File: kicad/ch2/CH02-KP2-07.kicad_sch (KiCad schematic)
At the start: 5 parts

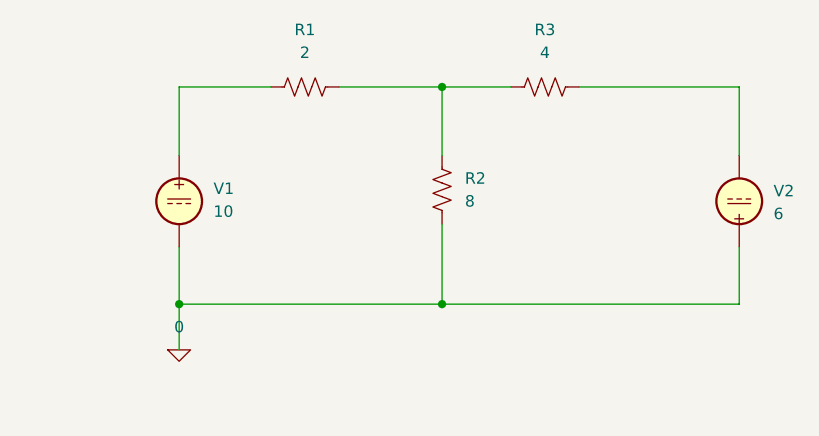
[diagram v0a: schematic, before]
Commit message: regular update
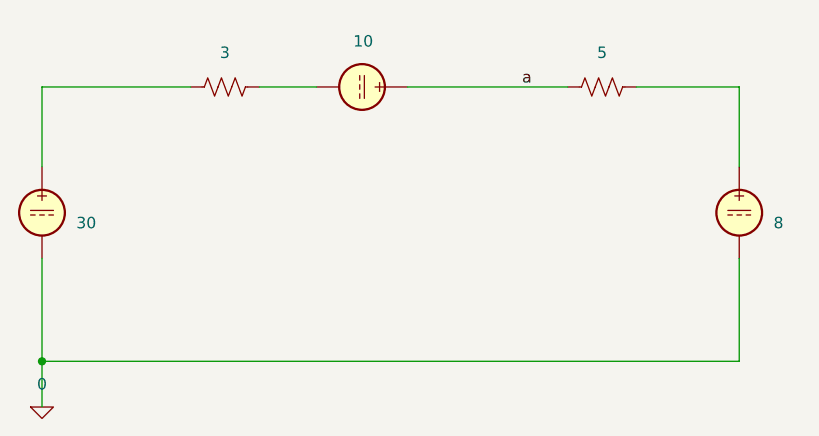
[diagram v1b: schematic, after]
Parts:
- removed R1: 2, symbol Device:R_US
- removed R2: 8, symbol Device:R_US
- removed R3: 4, symbol Device:R_US
- removed V1: 10, symbol Simulation_SPICE:VDC
- removed V2: 6, symbol Simulation_SPICE:VDC
- added R4: 3, symbol Device:R_US
- added R5: 5, symbol Device:R_US
- added V3: 30, symbol Simulation_SPICE:VDC
- added V4: 10, symbol Simulation_SPICE:VDC
- added V5: 8, symbol Simulation_SPICE:VDC
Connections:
- net 0: now also V3.2, V5.2
- new net: R5.2, V5.1
- new net: R4.2, V4.2
- new net: R4.1, V3.1
- new net a: R5.1, V4.1
